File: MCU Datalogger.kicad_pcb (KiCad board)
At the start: 4 copper layers, 28.8 x 36.2 mm, 29 parts, among them J1 Conn_01x04_Pin, J2 Conn_01x04_Pin, J3 Conn_01x09_Pin, J4 Conn_02x03_Odd_Even, U1 24LC1025, U2 24LC1025, U3 DS1337S_, U4 ATMEGA328P-AU, Y1 32.768 KHz, Y2 16 MHz

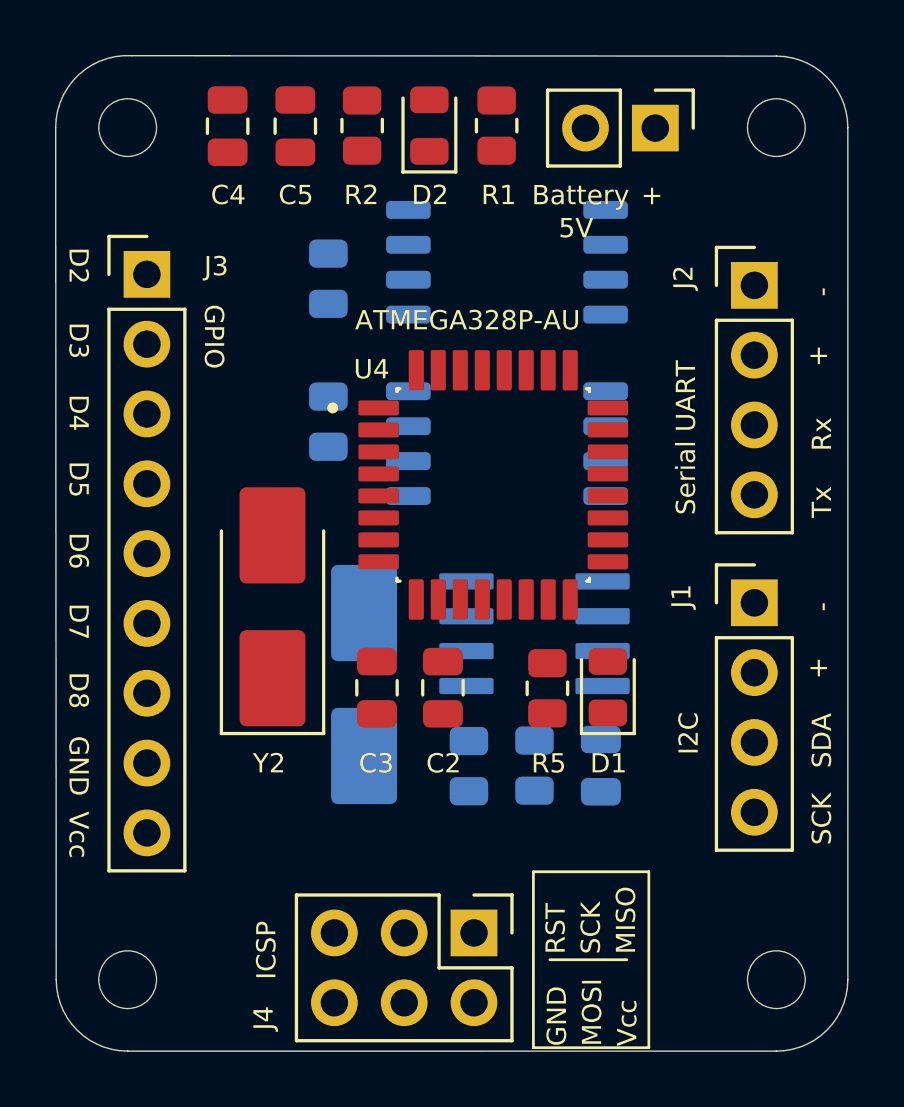
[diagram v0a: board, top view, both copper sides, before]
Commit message: route PCB
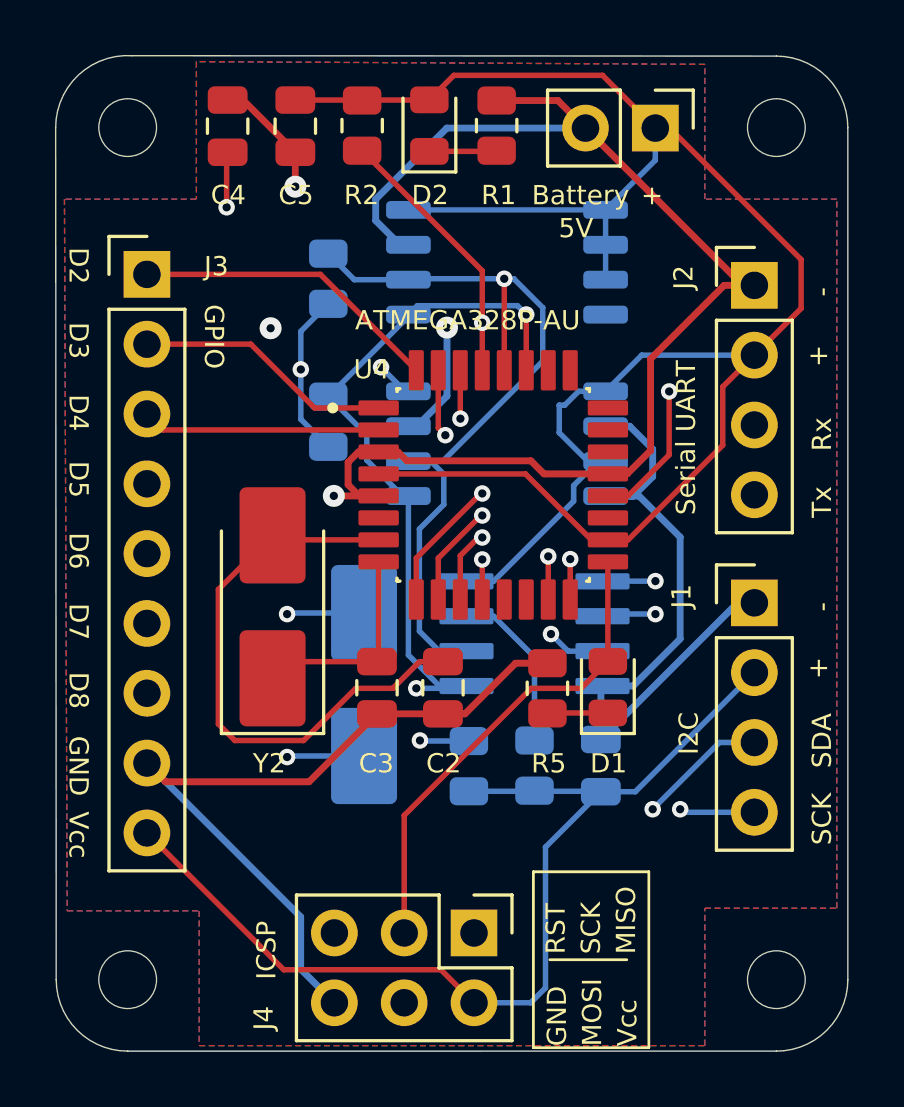
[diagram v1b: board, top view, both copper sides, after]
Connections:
- J1 pad 4: /SCK -> /SCL
- R3 pad 2: /SCK -> /SCL
- U1 pad 6: /SCK -> /SCL
- U2 pad 6: /SCK -> /SCL
- U3 pad 6: /SCK -> /SCL
- U4 pad 28: /SCK -> /SCL
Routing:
- net /Vcc: track 0.00 -> 143.1 mm, vias 0 -> 2
- net GND: track 0.00 -> 115.7 mm, vias 0 -> 4
- net /SCL: track 0.00 -> 55.6 mm, vias 0 -> 2
- net /SDA: track 0.00 -> 52.0 mm, vias 0 -> 3
- net /RESET: track 0.00 -> 37.1 mm, vias 0 -> 1
- net Net-(U4-AREF): track 0.00 -> 27.3 mm, vias 0 -> 2
- net Net-(U4-PB6): track 0.00 -> 21.2 mm
- net Net-(U3-X2): track 0.00 -> 20.3 mm, vias 0 -> 2
- net /MOSI: track 0.00 -> 20.0 mm, vias 0 -> 1
- net /D5: track 0.00 -> 18.7 mm, vias 0 -> 1
- net Net-(U3-X1): track 0.00 -> 18.6 mm, vias 0 -> 2
- net /SCK: track 0.00 -> 17.6 mm
- net /MISO: track 0.00 -> 17.3 mm, vias 0 -> 1
- net /D6: track 0.00 -> 16.5 mm, vias 0 -> 1
- net /D7: track 0.00 -> 16.2 mm, vias 0 -> 1
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- added copper zone on F.Cu, net /Vcc
- added copper zone on B.Cu, net GND
